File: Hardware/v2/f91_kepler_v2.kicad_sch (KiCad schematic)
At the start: 89 parts, among them J1 LS013B7DH03 FPC, Q1 FS8205A, SW1 BTN1/BSL, SW2 BTN2, SW3 BTN3, U1 CC2652R7RGZ, U2 BQ51050B, U3 DW01A, U4 XC6206P302MR, U5 LIS2DW12, U6 DRV2605L, U7 ST25DV04K, Y1 48MHz FA-128, Y2 32.768kHz FC-135

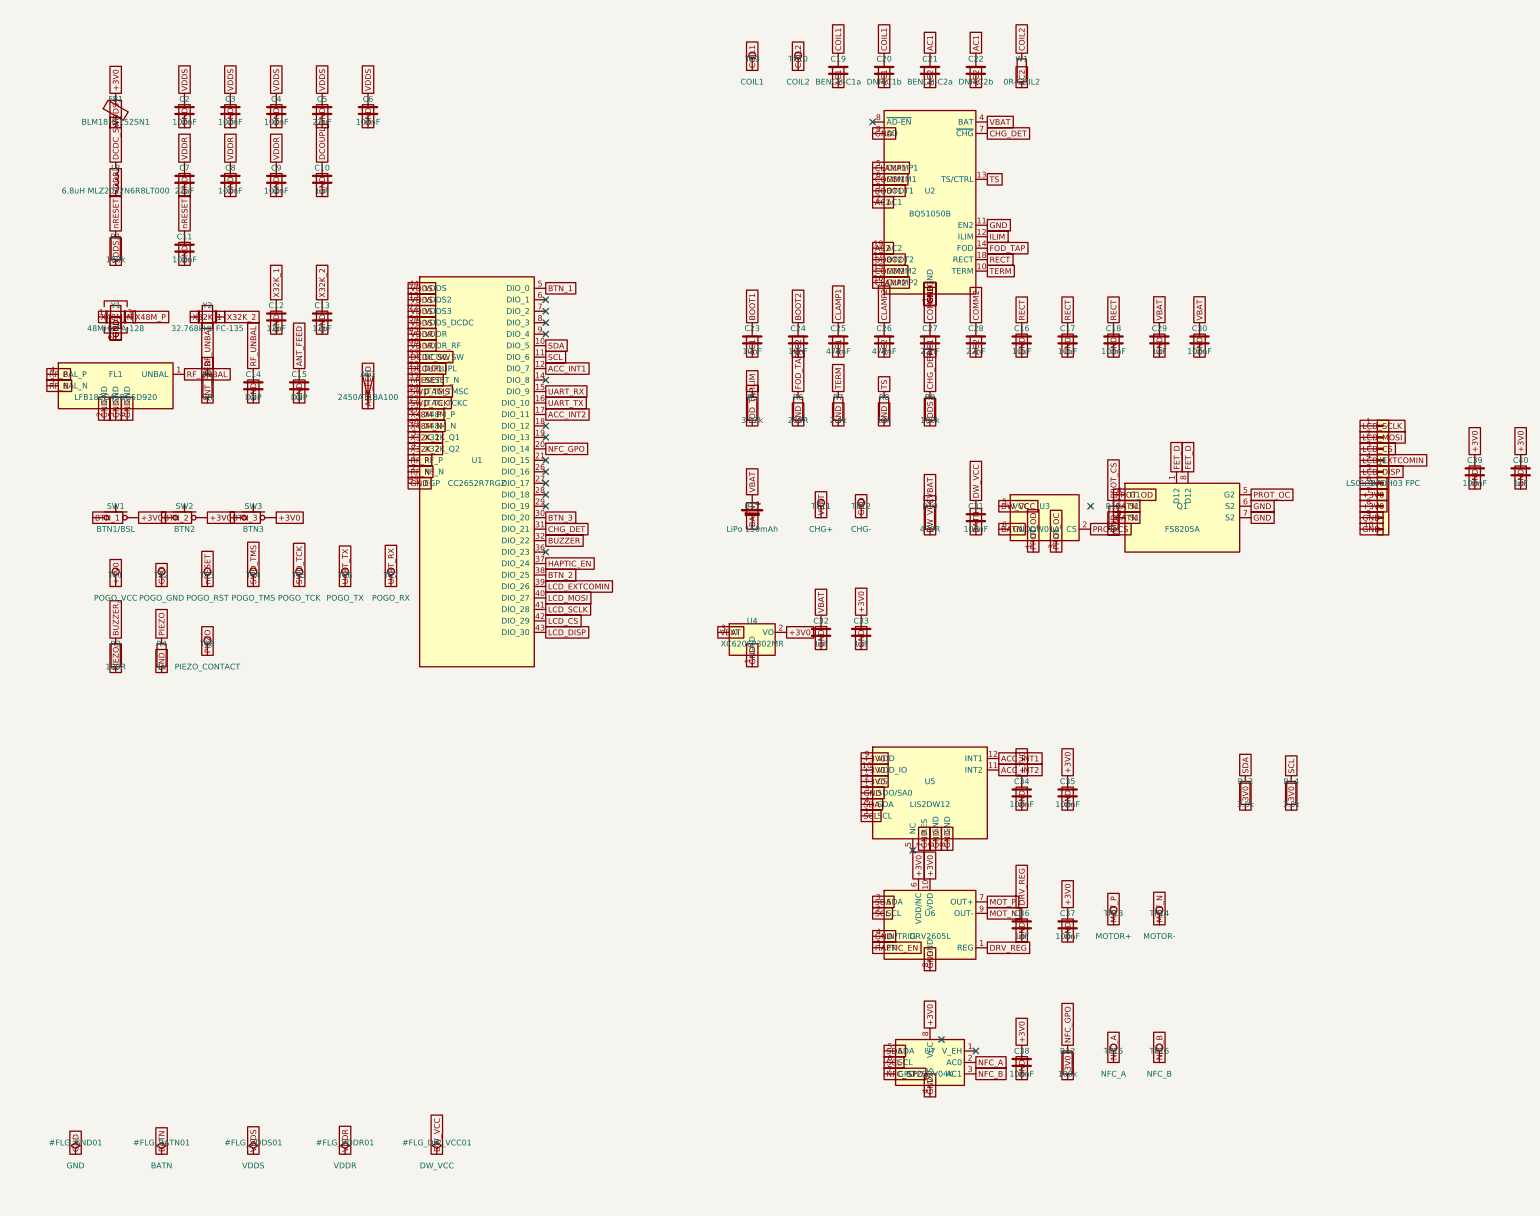
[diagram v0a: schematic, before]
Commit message: wip: snapshot pre-migración
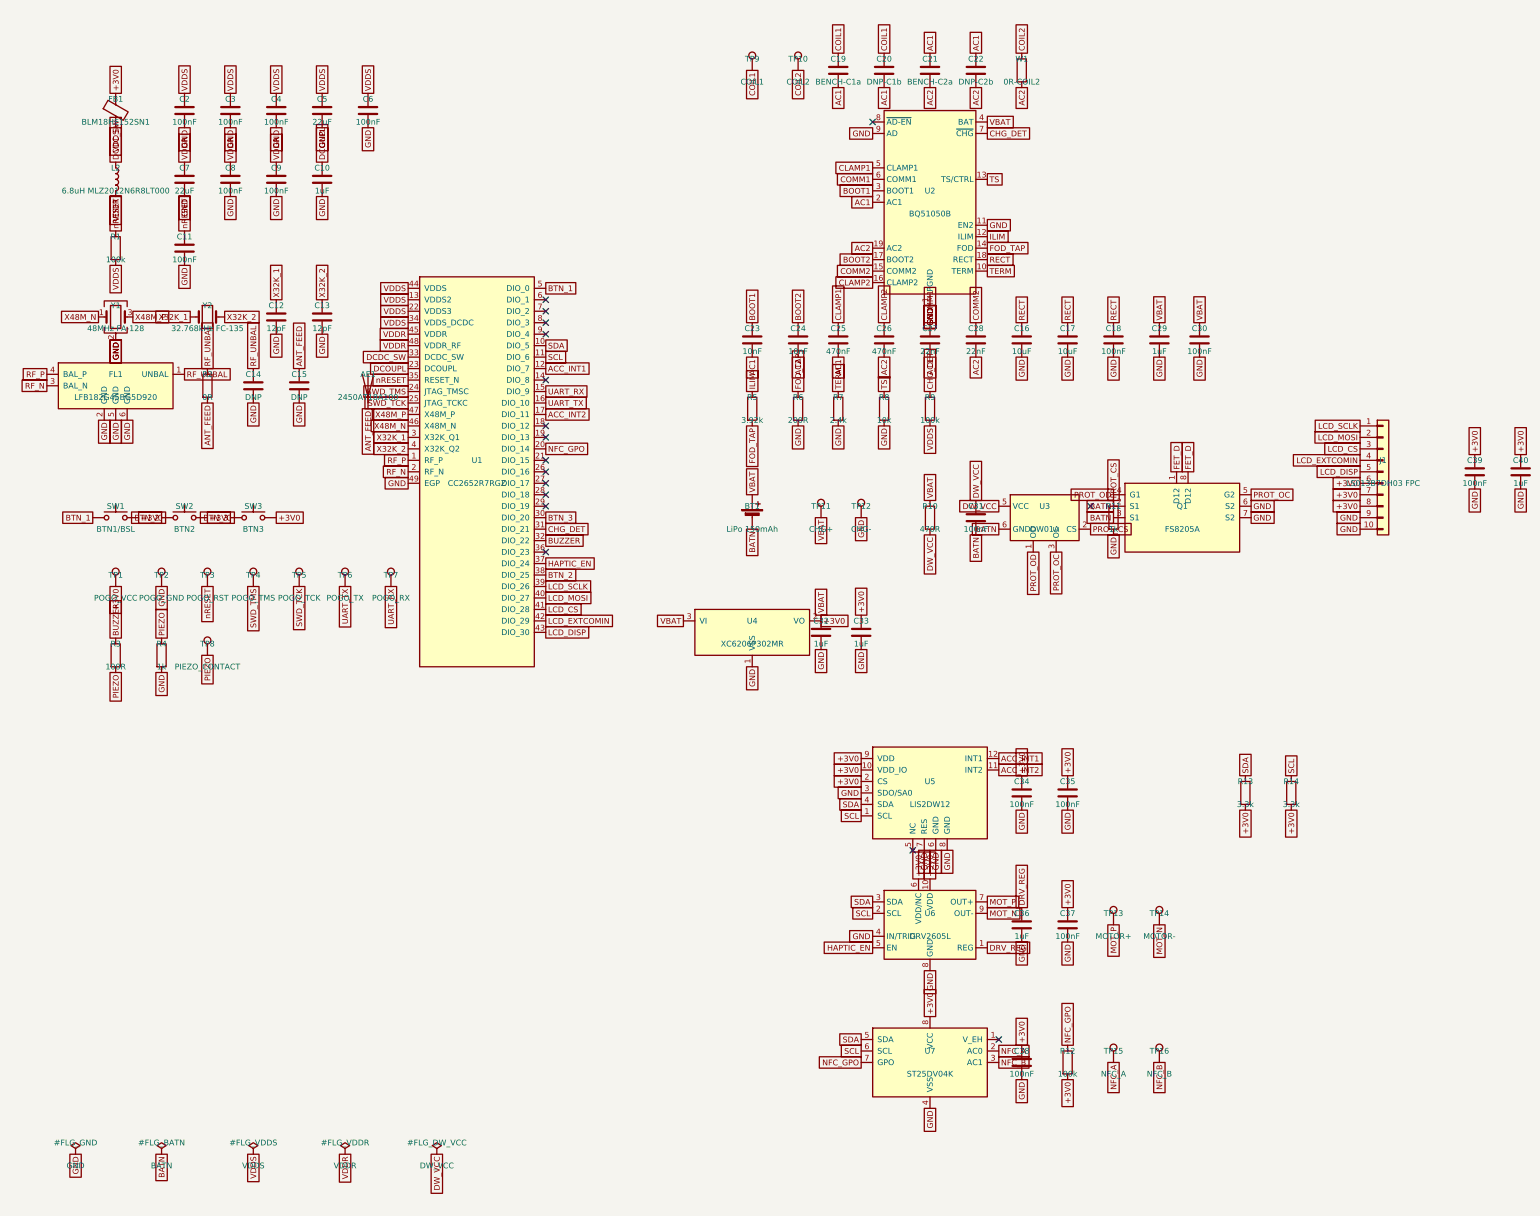
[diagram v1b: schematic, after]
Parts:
- removed U4: XC6206P302MR, Package_TO_SOT_SMD:SOT-23, symbol Regulator_Linear:XC6206PxxxMR
- removed U7: ST25DV04K, Package_SO:SOIC-8_3.9x4.9mm_P1.27mm, symbol RF_NFC:ST25DV04K-IER8C3
- added U4: XC6206P302MR, f91_footprints:Back_SOT-23, symbol f91:XC6206PxxxMR_F91
- added U7: ST25DV04K, f91_footprints:Back_SOIC-8_3.9x4.9mm_P1.27mm, symbol f91:ST25DV04K_SO8
- BT1: footprint f91_footprints:BatteryPads -> f91_footprints:Back_BatteryPads
- C16, C17, C19, C20: footprint Capacitor_SMD:C_0603_1608Metric -> f91_footprints:Back_C_0603_1608Metric
- C18, C21, C22, C23, C24, C25, C26, C27, C28, C29, C30, C31, C32, C33, C36, C37, C38: footprint Capacitor_SMD:C_0402_1005Metric -> f91_footprints:Back_C_0402_1005Metric
- FL1: footprint f91_footprints:Murata_LFB18_1608 -> f91_footprints:F91_Murata_LFB18_1608
- J1: footprint Connector_FFC-FPC:Hirose_FH12-10S-0.5SH_1x10-1MP_P0.50mm_Horizontal -> f91_footprints:F91_LCD_FPC_Hirose_FH12-10
- Q1: footprint Package_SO:TSSOP-8_3x3mm_P0.65mm -> f91_footprints:Back_TSSOP-8_3x3mm_P0.65mm
- R10, R11, R12, R13, R14, R5, R6, R7, R8, W1: footprint Resistor_SMD:R_0402_1005Metric -> f91_footprints:Back_R_0402_1005Metric
- TP1, TP10, TP11, TP12, TP13, TP14, TP15, TP16, TP2, TP3, TP4, TP5, TP6, TP7, TP8, TP9: footprint TestPoint:TestPoint_Pad_1.5x1.5mm -> f91_footprints:Back_TestPoint_Pad_1.5x1.5mm
- U2: footprint f91_footprints:VQFN-20-1EP_4.5x3.5mm_P0.5mm -> f91_footprints:Back_VQFN-20-1EP_4.5x3.5mm_P0.5mm
- U3: footprint Package_TO_SOT_SMD:SOT-23-6 -> f91_footprints:Back_SOT-23-6
- U6: footprint f91_footprints:VSSOP-10_3x3mm_P0.5mm -> f91_footprints:Back_VSSOP-10_3x3mm_P0.5mm
- Y1: footprint f91_footprints:Crystal_SMD_3215-4Pin_3.2x1.5mm -> f91_footprints:Epson_FA-128_2.0x1.6mm
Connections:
- net +3V0: now also U4.2 (VO), U7.8 (VCC)
- net GND: now also U4.1 (VSS), U7.4 (VSS)
- net LCD_CS: now also U1.41 (DIO_28); no longer U1.42 (DIO_29)
- net LCD_EXTCOMIN: now also U1.42 (DIO_29); no longer U1.39 (DIO_26)
- net LCD_SCLK: now also U1.39 (DIO_26); no longer U1.41 (DIO_28)
- net NFC_A: now also U7.2 (AC0)
- net NFC_B: now also U7.3 (AC1)
- net NFC_GPO: now also U7.7 (GPO)
- net SCL: now also U7.6 (SCL)
- net SDA: now also U7.5 (SDA)
- net VBAT: now also U4.3 (VI)
- no-connect marks 18 -> 17
